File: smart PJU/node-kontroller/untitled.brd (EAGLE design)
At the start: 80 x 80 mm, 50 parts, among them J1 U.FL-R-SMT(01), J2 10118193-0001LF, K2 SRD-05VDC-SL-C, Q1 S9013, Q16 MMBT3904, Q17 MMBT3904, Q18 12MHz, U1 AMS1117, U19 CH340G, U2 PC817X2NIP0F

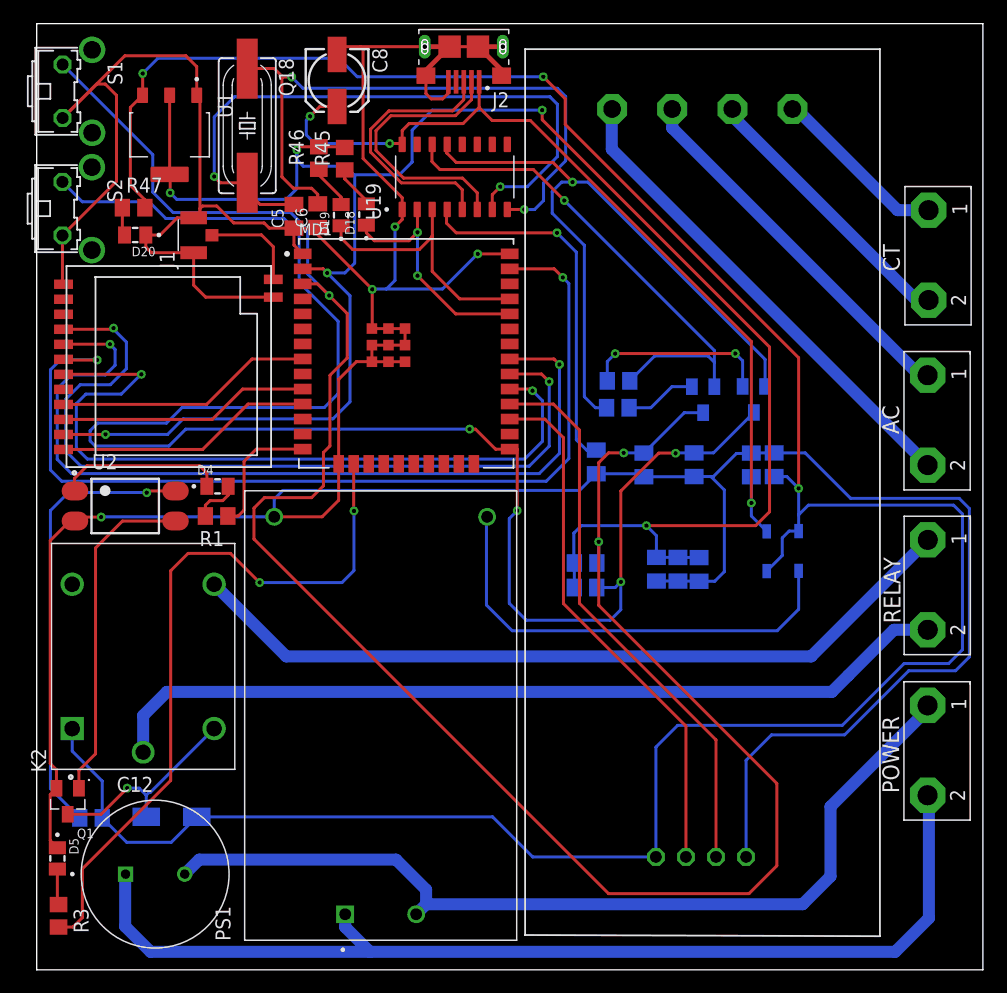
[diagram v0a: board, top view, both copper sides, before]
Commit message: revisi rangkaian
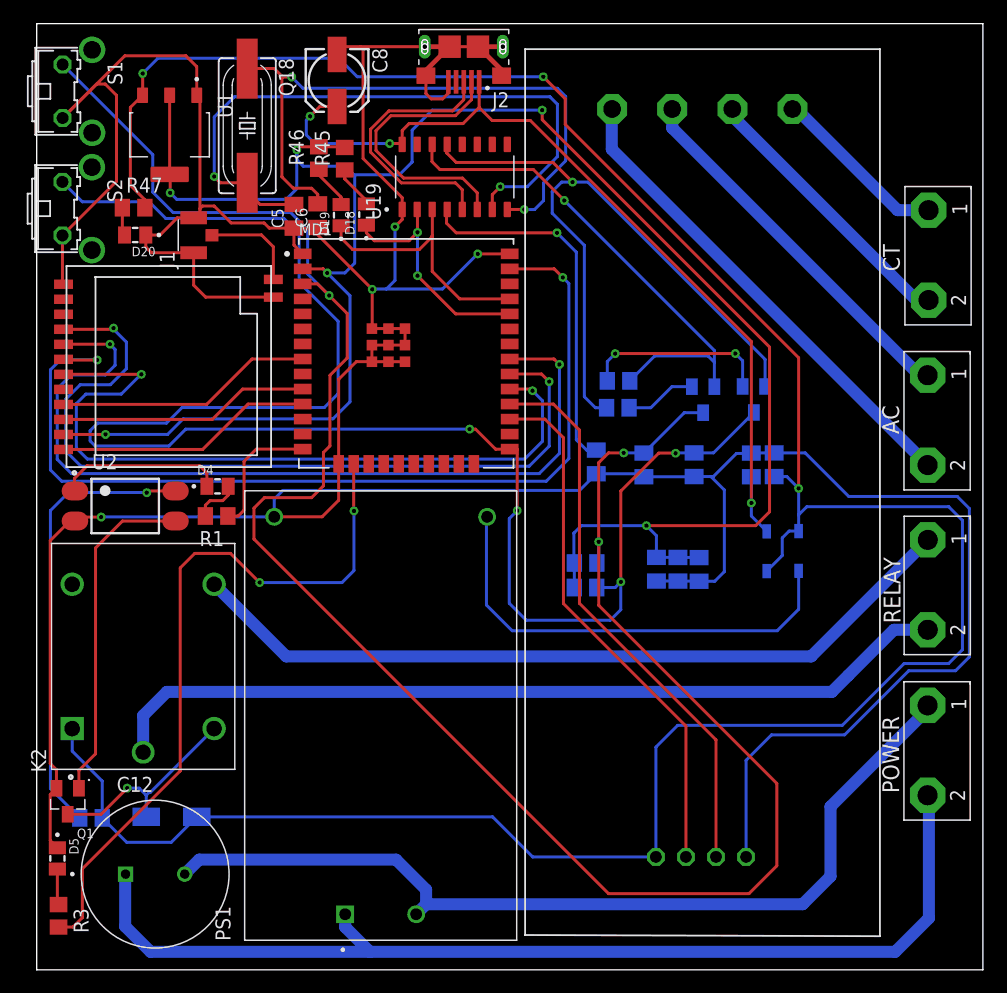
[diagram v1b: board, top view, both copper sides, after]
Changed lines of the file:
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@@
 <setting verticaltext="up"/>
 </settings>
-<grid distance="0.003125" unitdist="mic" unit="mm" style="lines" multiple="1" display="yes" altdistance="5" altunitdist="mil" altunit="mil"/>
+<grid distance="0.5" unitdist="mm" unit="mm" style="lines" multiple="1" display="yes" altdistance="5" altunitdist="mil" altunit="mil"/>
 <layers>
 <layer number="1" name="Top" color="4" fill="1" visible="yes" active="yes"/>
@@
 <wire x1="73.338565625" y1="25.897153125" x2="77.102621875" y2="25.897153125" width="0.254" layer="16"/>
 <wire x1="77.102621875" y1="25.897153125" x2="78.27220625" y2="27.0667375" width="0.254" layer="16"/>
-<wire x1="78.27220625" y1="27.0667375" x2="78.27220625" y2="38.539134375" width="0.254" layer="16"/>
-<wire x1="78.27220625" y1="38.539134375" x2="77.521609375" y2="39.28973125" width="0.254" layer="16"/>
-<wire x1="77.521609375" y1="39.28973125" x2="65.242903125" y2="39.28973125" width="0.254" layer="16"/>
-<wire x1="65.242903125" y1="39.28973125" x2="64.421646875" y2="38.468475" width="0.254" layer="16"/>
+<wire x1="78.27220625" y1="27.0667375" x2="78.27220625" y2="38.0002375" width="0.254" layer="16"/>
+<wire x1="78.27220625" y1="38.0002375" x2="77.113796875" y2="39.158646875" width="0.254" layer="16"/>
+<wire x1="77.113796875" y1="39.158646875" x2="65.11181875" y2="39.158646875" width="0.254" layer="16"/>
+<wire x1="65.11181875" y1="39.158646875" x2="64.421646875" y2="38.468475" width="0.254" layer="16"/>
 <wire x1="5.541034375" y1="12.848734375" x2="7.60865625" y2="10.7811125" width="0.254" layer="16"/>
 <wire x1="11.3760625" y1="10.7811125" x2="13.53185625" y2="12.93690625" width="0.254" layer="16"/>
@@
 <wire x1="77.686790625" y1="25.287809375" x2="78.857" y2="26.45801875" width="0.254" layer="16"/>
 <wire x1="78.857" y1="26.45801875" x2="78.857" y2="39.002490625" width="0.254" layer="16"/>
-<wire x1="78.857" y1="39.002490625" x2="77.99658125" y2="39.862909375" width="0.254" layer="16"/>
-<wire x1="77.99658125" y1="39.862909375" x2="68.821690625" y2="39.862909375" width="0.254" layer="16"/>
+<wire x1="78.857" y1="39.002490625" x2="77.83636875" y2="40.023121875" width="0.254" layer="16"/>
+<wire x1="77.83636875" y1="40.023121875" x2="68.661478125" y2="40.023121875" width="0.254" layer="16"/>
 <wire x1="64.979278125" y1="43.705321875" x2="62.35489375" y2="43.705321875" width="0.254" layer="16"/>
-<wire x1="68.821690625" y1="39.862909375" x2="64.979278125" y2="43.705321875" width="0.254" layer="16"/>
+<wire x1="68.661478125" y1="40.023121875" x2="64.979278125" y2="43.705321875" width="0.254" layer="16"/>
 <wire x1="55.583725" y1="41.70909375" x2="57.004628125" y2="41.70909375" width="0.254" layer="16"/>
 <wire x1="57.004628125" y1="41.70909375" x2="57.212775" y2="41.70909375" width="0.254" layer="16"/>
@@
 <wire x1="21.750346875" y1="62.711228125" x2="19.664753125" y2="62.711228125" width="0.254" layer="1"/>
 <wire x1="19.664753125" y1="62.711228125" x2="19.22711875" y2="63.1488625" width="0.254" layer="1"/>
-<wire x1="19.22711875" y1="63.1488625" x2="16.6598375" y2="63.1488625" width="0.254" layer="1"/>
-<wire x1="16.6598375" y1="63.1488625" x2="15.226446875" y2="64.582253125" width="0.254" layer="1"/>
+<wire x1="19.22711875" y1="63.1488625" x2="16.441365625" y2="63.1488625" width="0.254" layer="1"/>
+<wire x1="16.441365625" y1="63.1488625" x2="15.007975" y2="64.582253125" width="0.254" layer="1"/>
 <wire x1="13.529525" y1="73.9466875" x2="13.529525" y2="76.3655125" width="0.254" layer="1"/>
 <wire x1="13.529525" y1="76.3655125" x2="12.609725" y2="77.2853125" width="0.254" layer="1"/>
@@
 <wire x1="34.9094125" y1="78.05365" x2="37.3191875" y2="78.05365" width="0.254" layer="1"/>
 <wire x1="14.02280625" y1="64.582253125" x2="13.80331875" y2="64.362765625" width="0.254" layer="1"/>
-<wire x1="15.226446875" y1="64.582253125" x2="14.02280625" y2="64.582253125" width="0.254" layer="1"/>
+<wire x1="15.007975" y1="64.582253125" x2="14.02280625" y2="64.582253125" width="0.254" layer="1"/>
 <wire x1="1.669653125" y1="15.352003125" x2="1.669653125" y2="16.917603125" width="0.254" layer="1"/>
 <wire x1="1.669653125" y1="16.917603125" x2="1.143" y2="17.44425625" width="0.254" layer="1"/>
@@
 <wire x1="3.06565625" y1="3.61890625" x2="3.859878125" y2="4.413128125" width="0.254" layer="1"/>
 <wire x1="3.859878125" y1="4.413128125" x2="3.859878125" y2="8.543721875" width="0.254" layer="1"/>
-<wire x1="3.859878125" y1="8.543721875" x2="11.327715625" y2="16.011559375" width="0.254" layer="1"/>
-<wire x1="11.327715625" y1="16.011559375" x2="11.327715625" y2="33.740859375" width="0.254" layer="1"/>
-<wire x1="11.327715625" y1="33.740859375" x2="12.796546875" y2="35.209690625" width="0.254" layer="1"/>
-<wire x1="12.796546875" y1="35.209690625" x2="16.384671875" y2="35.209690625" width="0.254" layer="1"/>
+<wire x1="3.859878125" y1="8.543721875" x2="12.133284375" y2="16.817128125" width="0.254" layer="1"/>
+<wire x1="12.133284375" y1="16.817128125" x2="12.133284375" y2="33.980696875" width="0.254" layer="1"/>
+<wire x1="12.133284375" y1="33.980696875" x2="13.362278125" y2="35.209690625" width="0.254" layer="1"/>
+<wire x1="13.362278125" y1="35.209690625" x2="16.384671875" y2="35.209690625" width="0.254" layer="1"/>
 <wire x1="16.384671875" y1="35.209690625" x2="18.8504375" y2="32.743925" width="0.254" layer="1"/>
 <via x="18.8504375" y="32.743925" extent="1-16" drill="0.35"/>
